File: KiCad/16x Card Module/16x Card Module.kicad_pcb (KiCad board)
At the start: 4 copper layers, 75 x 100 mm, 46 parts, among them J1 Conn_02x25_Odd_Even, J2 Conn_ARM_SWD_TagConnect_TC2030, U1 STM32F411RETx, U2 D1213A-04S-7, U3 D1213A-04S-7, U4 D1213A-04S-7, U5 D1213A-04S-7, U6 D1213A-04S-7, U7 74LVC1G126, U8 74LVC1G126, X1 16Mhz

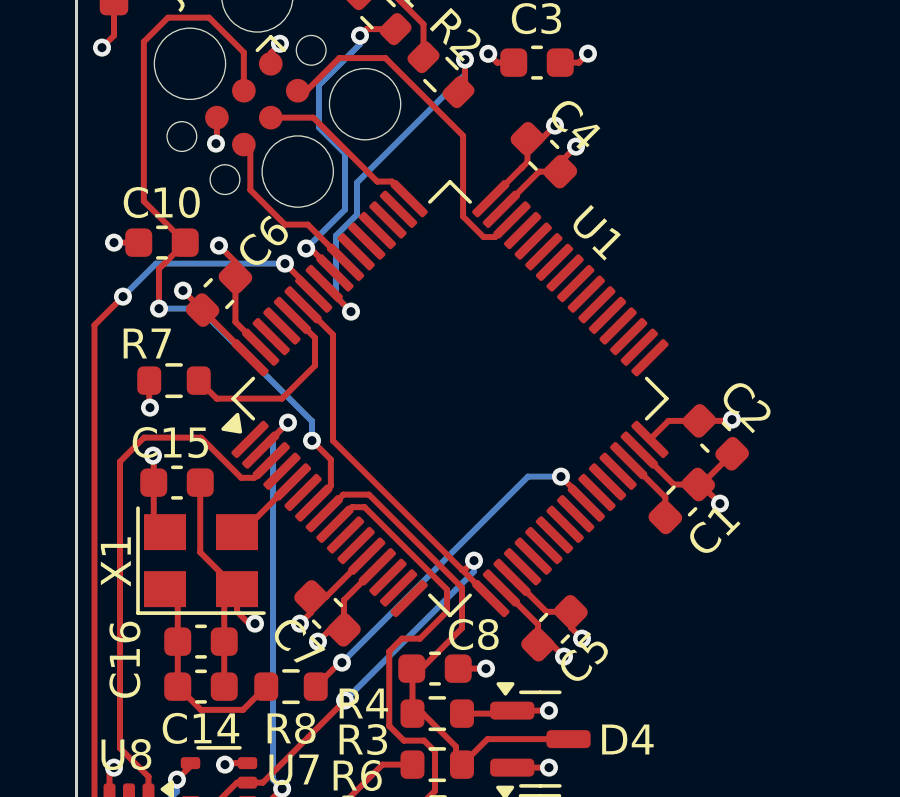
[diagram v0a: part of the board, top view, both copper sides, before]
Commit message: update
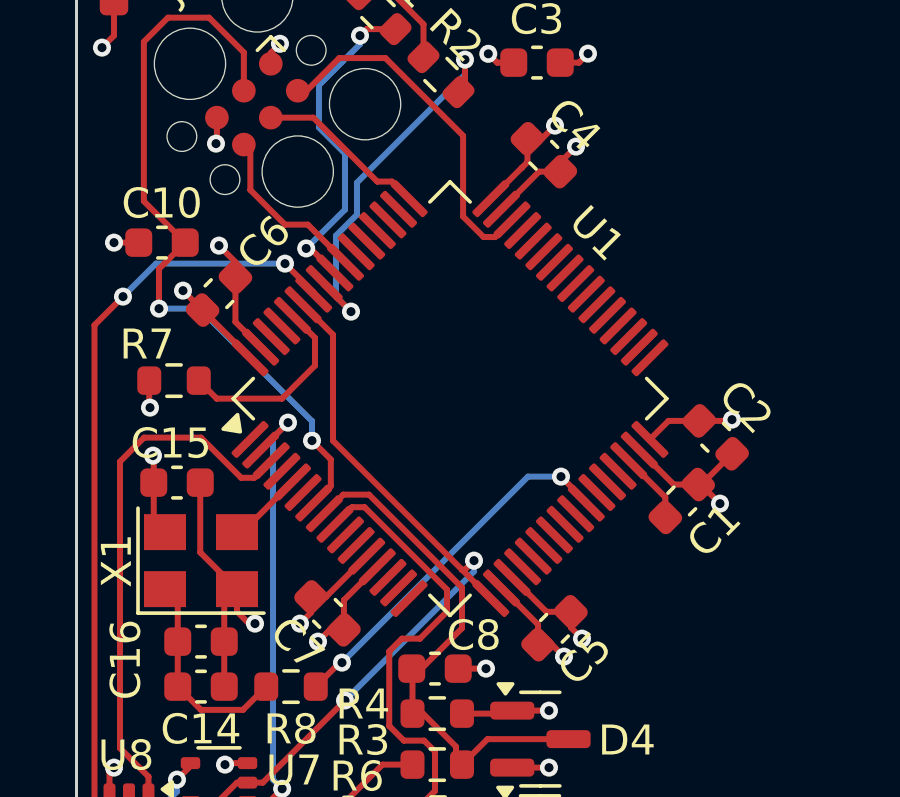
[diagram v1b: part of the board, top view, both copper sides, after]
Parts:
- U1: footprint Package_QFP:LQFP-64_10x10mm_P0.5mm -> footprints:LQFP-64_10x10mm_P0.5mm_smaller_pads
- X1: value 16Mhz -> 25Mhz
